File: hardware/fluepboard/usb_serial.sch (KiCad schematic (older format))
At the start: 13 parts, among them U3 CP2102N-A01-GQFN24

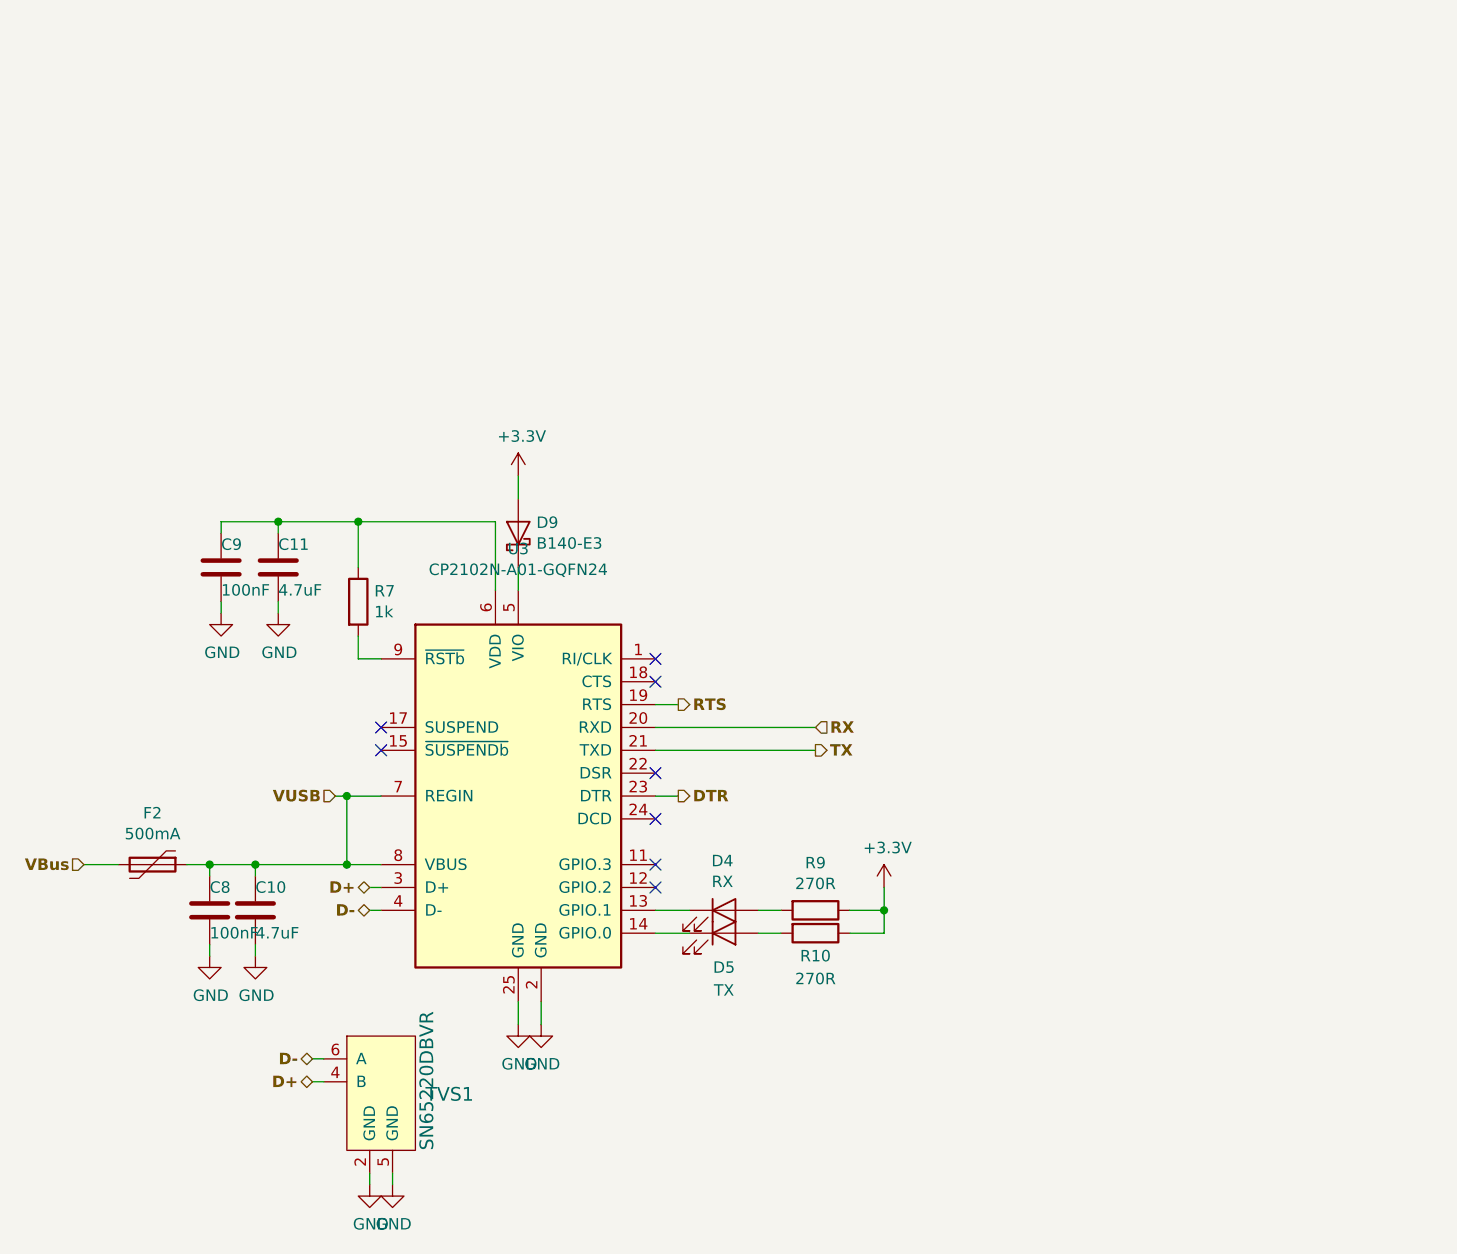
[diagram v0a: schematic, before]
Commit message: Commit jlcpcb compatible version
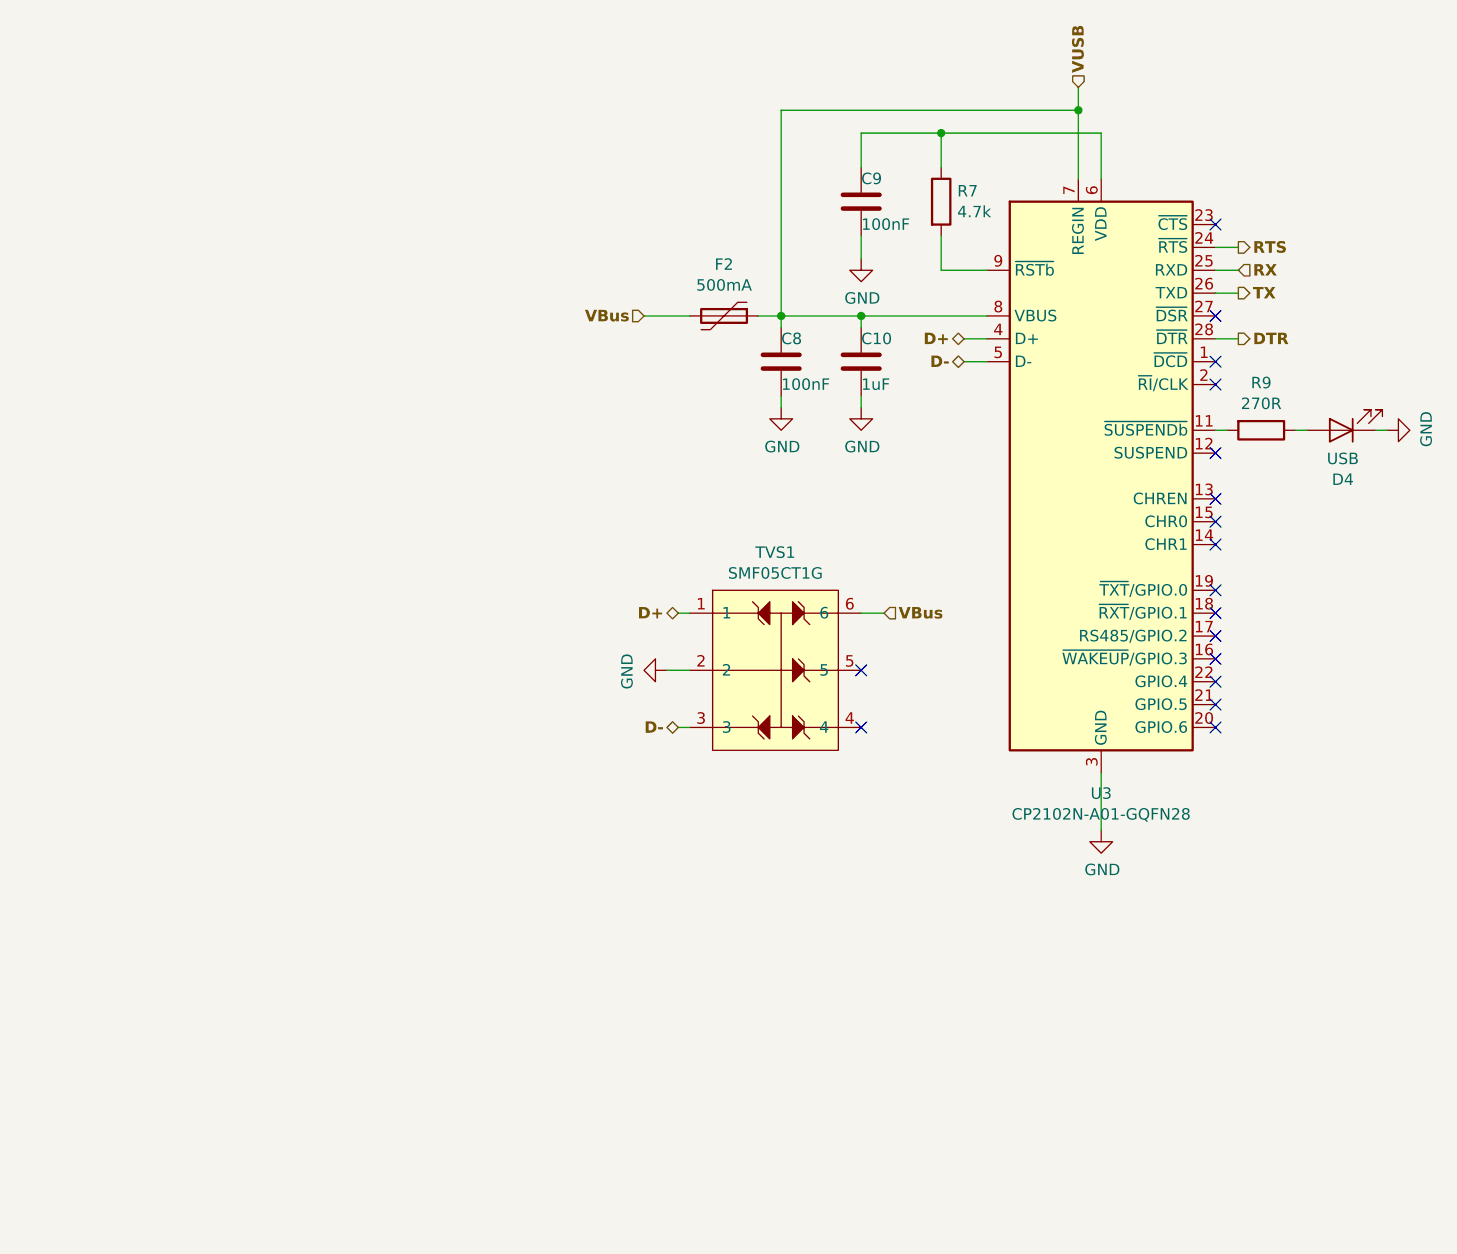
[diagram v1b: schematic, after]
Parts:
- removed C11: 4.7uF, Capacitor_SMD:C_0805_2012Metric, symbol Device:C
- removed D5: TX, Diode_SMD:D_0805_2012Metric, symbol Device:LED
- removed D9: B140-E3, Diode_SMD:D_SMA, symbol Diode:B140-E3
- removed R10: 270R, Resistor_SMD:R_0805_2012Metric, symbol Device:R
- removed TVS1: SN65220DBVR, Package_TO_SOT_SMD:SOT-23-6, symbol dk_TVS-Mixed-Technology:SN65220DBVR
- removed U3: CP2102N-A01-GQFN24, Package_DFN_QFN:QFN-24-1EP_4x4mm_P0.5mm_EP2.6x2.6mm, symbol Interface_USB:CP2102N-A01-GQFN24
- added TVS1: SMF05CT1G, Package_TO_SOT_SMD:SOT-363_SC-70-6, symbol fluepdot:SMF05CT1G
- added U3: CP2102N-A01-GQFN28, Package_DFN_QFN:QFN-28-1EP_5x5mm_P0.5mm_EP3.35x3.35mm, symbol Interface_USB:CP2102N-A01-GQFN28
- C10: value 4.7uF -> 1uF; footprint Capacitor_SMD:C_0805_2012Metric -> Capacitor_SMD:C_0603_1608Metric; Description (none) -> MULTILAYER CERAMIC CAPACITORS MLCC - SMD/SMT 1UF 50V 0603 R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; Extended Part (none) -> 0; LCSC (none) -> C15849; Manufacturer (none) -> CL10A105KB8NNNC; Octopart C0805C475K3PAC -> (none)
- C8, C9: footprint Capacitor_SMD:C_0805_2012Metric -> Capacitor_SMD:C_0603_1608Metric; Description (none) -> MULTILAYER CERAMIC CAPACITORS MLCC - SMD/SMT 100NF 50V 0603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; Extended Part (none) -> 0; LCSC (none) -> C14663; Manufacturer (none) -> CC0603KRX7R9BB104
- D4: value RX -> USB; Description (none) -> LIGHT EMITTING DIODES (LED) YELLOW 592~594NM 95~113MCD@20MA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; Extended Part (none) -> 0; LCSC (none) -> C2296; Manufacturer (none) -> 17-21SUYC/TR8
- F2: Description (none) -> PTC RESETTABLE FUSES 1206 ROHS; Extended Part (none) -> 1; LCSC (none) -> C69688; Manufacturer (none) -> nSMD050
- R7: value 1k -> 4.7k; footprint Resistor_SMD:R_0805_2012Metric -> Resistor_SMD:R_0603_1608Metric; Description (none) -> CHIP RESISTOR - SURFACE MOUNT 4.7KOHMS ±1% 1/10W 0603 ROHS; Extended Part (none) -> 0; LCSC (none) -> C23162; Manufacturer (none) -> 0603WAF4701T5E; Octopart RC0805FR-071K -> (none)
- R9: footprint Resistor_SMD:R_0805_2012Metric -> Resistor_SMD:R_0603_1608Metric; Description (none) -> CHIP RESISTOR - SURFACE MOUNT 270OHMS ±1% 1/10W 0603 ROHS; Extended Part (none) -> 0; LCSC (none) -> C22966; Manufacturer (none) -> 0603WAF2700T5E
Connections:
- net +3V3 is gone; now on an unnamed net: R9.1
- net D+: now also TVS1.1, U3.4 (D+)
- net D-: now also TVS1.3, U3.5 (D-)
- net DTR: now also U3.28 (~DTR)
- net GND: now also D4.1 (K), TVS1.2, U3.29 (GND), U3.3 (GND)
- net RTS: now also U3.24 (~RTS)
- net RX: now also U3.25 (RXD)
- net TX: now also U3.26 (TXD)
- net VBus: now also TVS1.6
- net VUSB: now also U3.7 (REGIN), U3.8 (VBUS)
- net at D4.2 (A): no longer R9.2
- net at C9.2, R7.1: now also U3.6 (VDD)
- net at R7.2: now also U3.9 (~RSTb)
- new net: R9.2, U3.11 (~SUSPENDb)
- no-connect marks 8 -> 17
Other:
- moved on the sheet: C10, C8, C9, D4, F2, R7, R9
